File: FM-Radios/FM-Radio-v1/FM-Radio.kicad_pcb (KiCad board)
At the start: 4 copper layers, 45.1 x 57 mm, 64 parts, among them IC1 TPS62160DGKR, J1 L_OUT, J2 USB_C_Receptacle_USB2.0, J3 R_OUT, J5 GND, J6 BWSMA-KE-Z001, J8 3V3, J9 VBUS, SW2 EN, U1 ESP32-S3-MINI-1U, U2 SI4702-C19-GMR, U4 PRTR5V0U2X, U6 PAM8406D, Y1 32.768 kHz

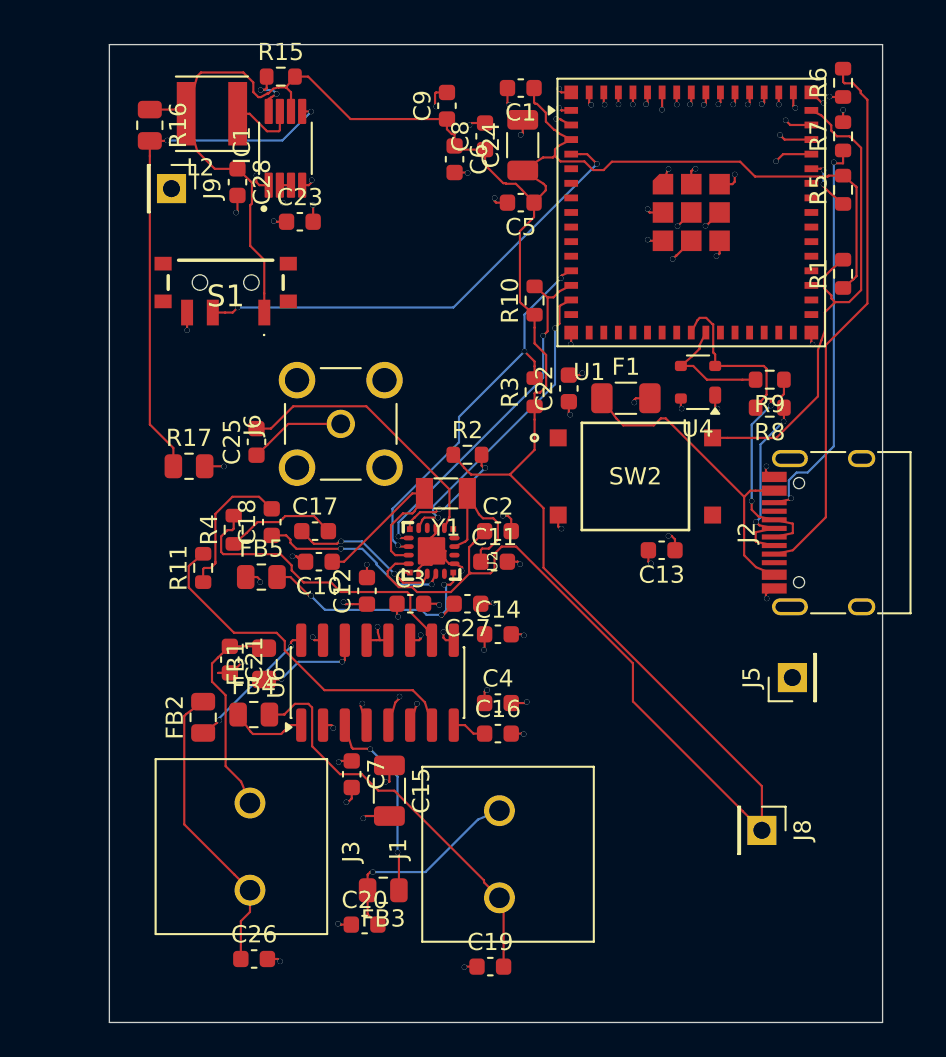
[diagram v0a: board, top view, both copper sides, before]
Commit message: Shenanigooner
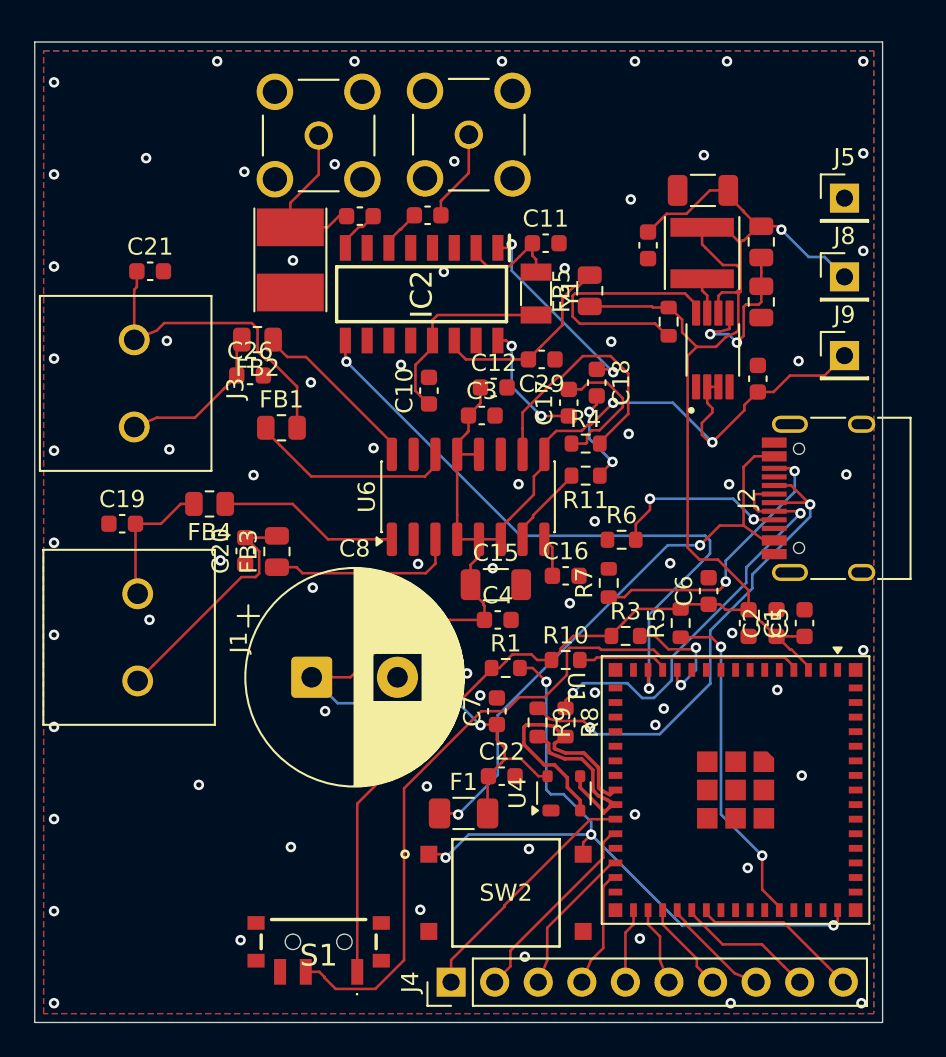
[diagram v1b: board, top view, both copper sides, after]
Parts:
- removed C13, C14, C9: 100nF, Capacitor_SMD:C_0603_1608Metric
- removed R2: 10k Ohm, Resistor_SMD:R_0603_1608Metric
- removed U2: SI4702-C19-GMR, footprints:SI470X_20_QFN
- added C29: 100nF, Capacitor_SMD:C_0603_1608Metric, F.Cu at (175.3, 101.5)
- added IC2: SI4732-A10-GSR, footprints:SOIC127P600X175-16N, F.Cu at (168.2, 97.7)
- added J4: Conn_01x10_Pin, Connector_PinHeader_2.54mm:PinHeader_1x10_P2.54mm_Vertical, F.Cu at (170.0, 137.8)
- added J7: AM-ANT, footprints:BAT_WIRELESS_BWSMA-KE-Z001, F.Cu at (162.2, 88.4)
- added L3: 500 uH, Inductor_SMD:L_Taiyo-Yuden_NR-40xx_HandSoldering, F.Cu at (160.6, 95.7)
- C27: value 10uF -> 470 nF
- C8: value 100nF -> 680 uF; footprint Capacitor_SMD:C_0603_1608Metric -> Capacitor_THT:CP_Radial_D12.5mm_P5.00mm
- J6: value BWSMA-KE-Z001 -> FM-ANT
- moved J9 40.4 mm to (192.9, 101.2), turned to 0 degrees
- moved S1 38.8 mm to (162.2, 135.4)
- moved R16 36.3 mm to (188.1, 94.6)
- moved R17 34.7 mm to (188.1, 98.1), turned to -90 degrees
- moved C26 34.0 mm to (158.3, 102.4)
- moved C1 33.9 mm to (187.3, 116.8), turned to -90 degrees
- moved U1 33.8 mm to (186.6, 126.5), turned to -90 degrees
- moved C19 33.6 mm to (150.8, 111.0)
- moved C8 33.1 mm to (161.8, 120.0), turned to 0 degrees
- moved J8 32.6 mm to (192.9, 96.6), turned to 0 degrees
- moved R1 30.2 mm to (173.2, 119.4), turned to 0 degrees
- moved L2 29.7 mm to (184.6, 95.2), turned to 90 degrees
- moved R6 29.6 mm to (179.9, 112.0), turned to 0 degrees
- moved C5 29.6 mm to (190.6, 116.8), turned to 90 degrees
- moved R7 29.4 mm to (179.2, 114.5)
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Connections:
- C25 pad 2: Net-(U2-FMIP) -> /FMI
- C27 pad 1: GND -> Net-(C27-Pad1)
- C27 pad 2: Net-(U2-VA) -> /AMI
- C8 pad 1: +3.3V -> +5V
- FB5 pad 1: +5V -> +3.3V
- FB5 pad 2: Net-(U2-VA) -> +3.3VA
- SW2 pad A: unconnected-(SW2-PadA) -> Net-(U1-EN)
- SW2 pad D: unconnected-(SW2-PadD) -> GND
- U1 pad 25: unconnected-(U1-IO21-Pad25) -> Net-(J4-Pin_1)
- U1 pad 26: unconnected-(U1-IO26-Pad26) -> Net-(J4-Pin_2)
- U1 pad 28: unconnected-(U1-IO33-Pad28) -> Net-(J4-Pin_3)
- U1 pad 29: unconnected-(U1-IO34-Pad29) -> Net-(J4-Pin_4)
- U1 pad 31: unconnected-(U1-IO35-Pad31) -> Net-(J4-Pin_5)
- U1 pad 32: unconnected-(U1-IO36-Pad32) -> Net-(J4-Pin_6)
- U1 pad 33: unconnected-(U1-IO37-Pad33) -> Net-(J4-Pin_7)
- U1 pad 34: unconnected-(U1-IO38-Pad34) -> Net-(J4-Pin_8)
- U1 pad 35: unconnected-(U1-IO39-Pad35) -> Net-(J4-Pin_9)
- U1 pad 36: unconnected-(U1-IO40-Pad36) -> Net-(J4-Pin_10)
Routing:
- net GND: track 75.0 -> 0.00 mm, vias 72 -> 71
- net +3.3V: track 166.3 -> 103.9 mm, vias 0 -> 1
- net +5V: track 21.2 -> 83.2 mm, vias 19 -> 3
- net Net-(J2-CC1): track 31.9 -> 10.5 mm, vias 0 -> 2
- net Net-(IC1-FB): track 30.2 -> 9.88 mm
- net /RST: track 17.8 -> 38.0 mm
- net /BOOTMODE: track 27.7 -> 44.4 mm, vias 2 -> 0
- net Net-(J2-D+-PadA6): track 12.8 -> 29.4 mm
- net Net-(U2-FMIP): track 16.1 -> 0.00 mm
- net Net-(U1-IO45): track 3.23 -> 19.3 mm
- net /GPIO8: track 23.0 -> 7.16 mm, vias 3 -> 2
- net Net-(J1-Pin_1): track 23.9 -> 8.01 mm
- net Net-(U6-INL): track 20.6 -> 4.81 mm
- net VBUS: track 18.6 -> 34.3 mm, vias 0 -> 2
- net /GPIO9: track 20.8 -> 5.28 mm, vias 2 -> 0
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- added copper zone on B.Cu, net GND
- added copper zone on F.Cu, net GND
- removed copper zone on In2.Cu, net +5V
- removed copper zone on In1.Cu, net GND
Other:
- board size 45.1 x 57 mm -> 49.4 x 57.1 mm
- copper layers 4 -> 2
